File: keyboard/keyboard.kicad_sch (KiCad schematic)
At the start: 64 parts, among them J1 Conn_01x04, J2 Conn_01x04, SW1 SW_Push, SW10 SW_Push, SW11 SW_Push, SW12 SW_Push, SW13 SW_Push, SW14 SW_Push, SW15 SW_Push, SW16 SW_Push, SW17 SW_Push, SW18 SW_Push, SW19 SW_Push, SW2 SW_Push, SW20 SW_Push, SW21 SW_Push, SW3 SW_Push, SW4 SW_Push, SW5 SW_Push, SW6 SW_Push, SW7 SW_Push, SW8 SW_Push, SW9 SW_Push, U1 AP2127K-3.3, U2 USBLC6-2SC6, U3 STM32F072CBTx

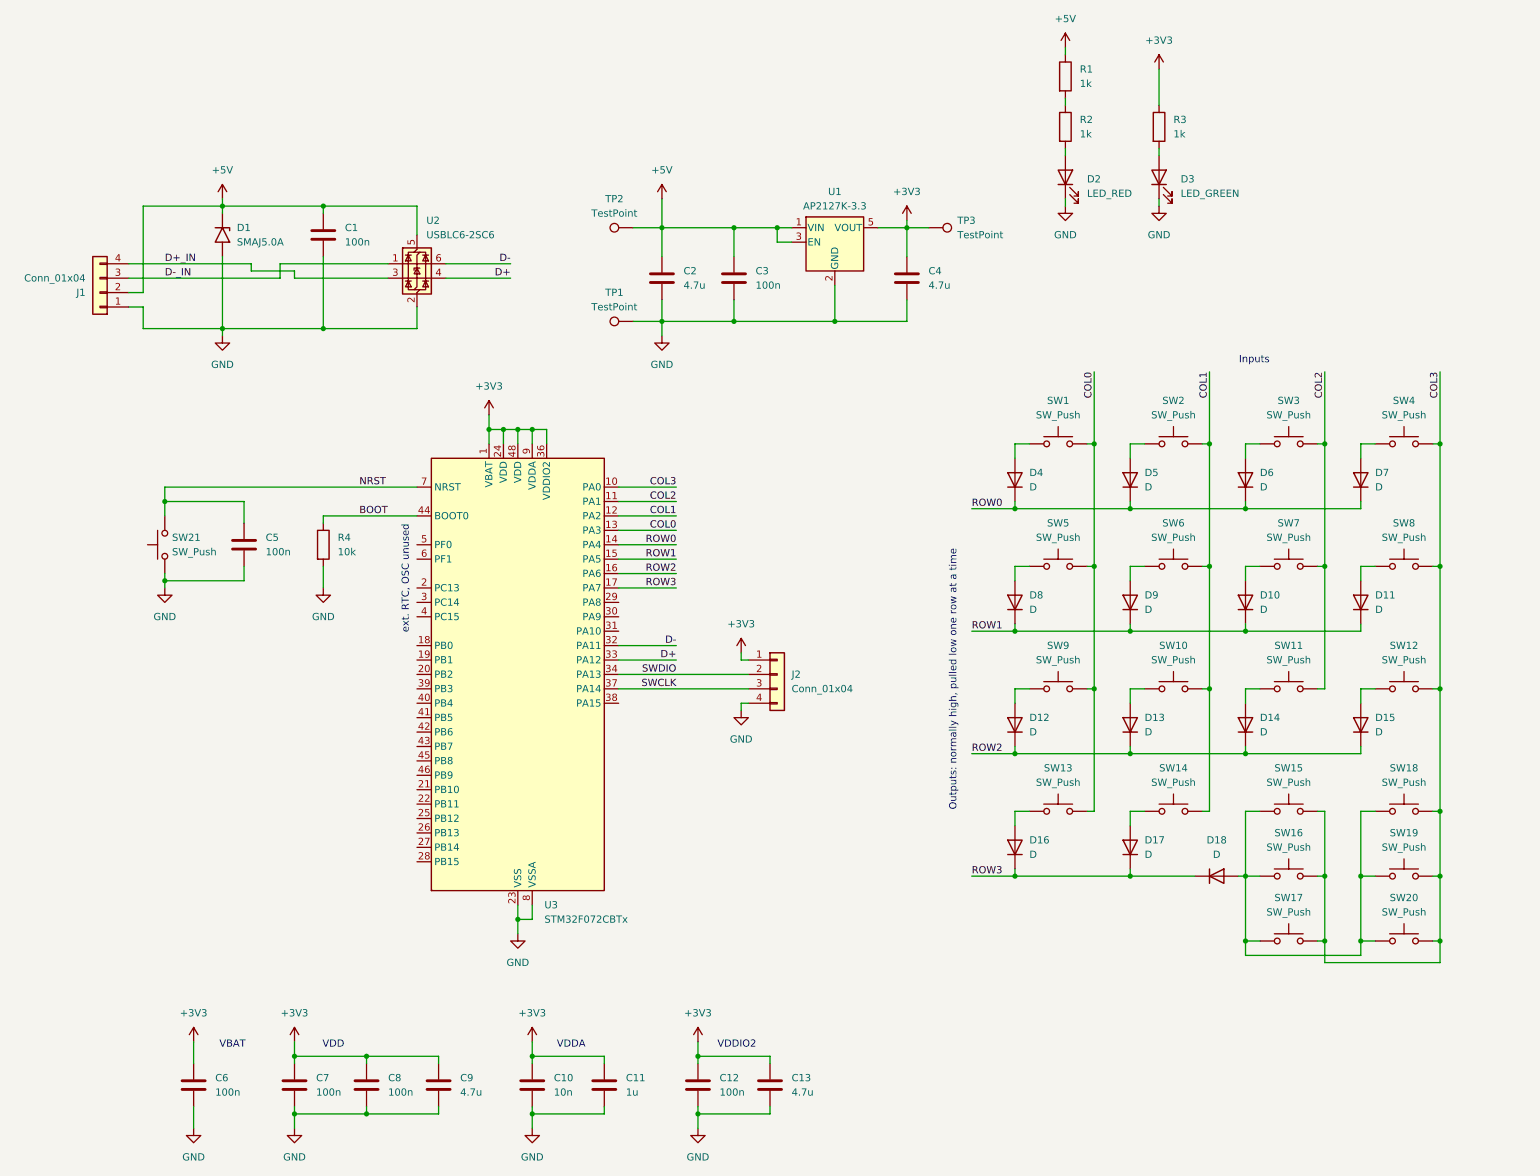
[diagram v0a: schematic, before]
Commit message: Some routing.
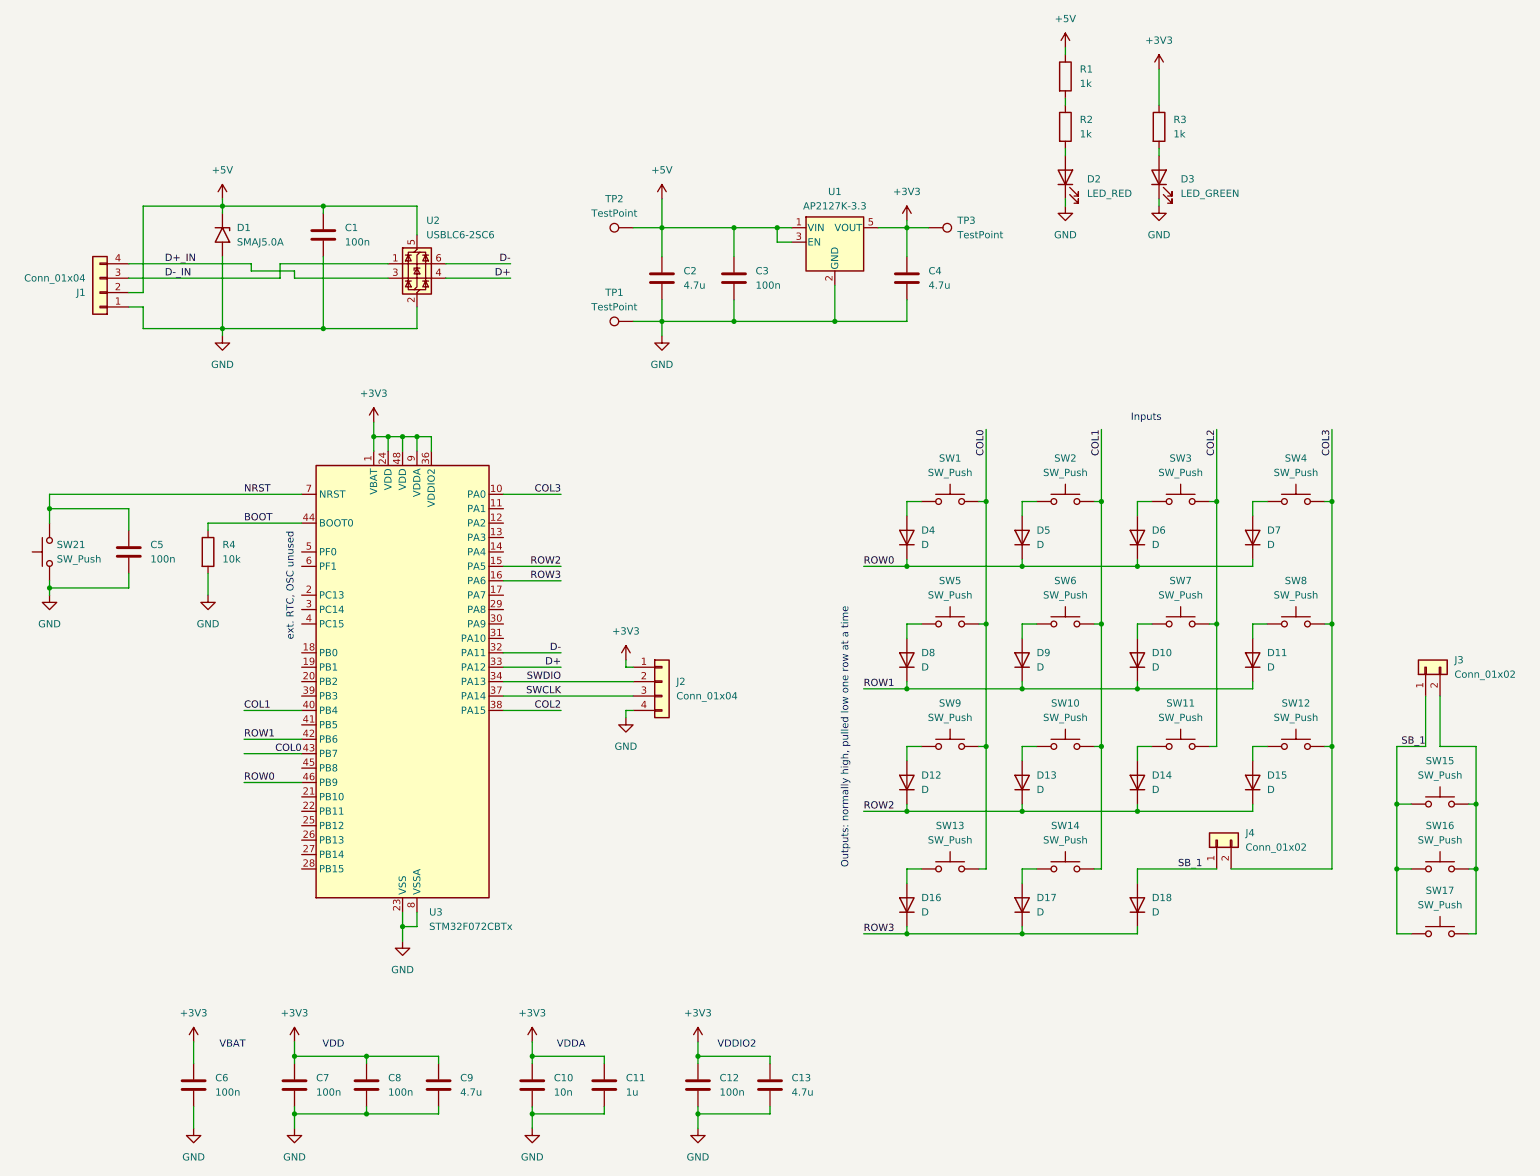
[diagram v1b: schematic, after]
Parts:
- removed SW18, SW19, SW20: SW_Push, PCM_marbastlib-mx:SW_MX_HS_KS-2P02B01-01_1.5u, symbol Switch:SW_Push
- added J3, J4: Conn_01x02, symbol Connector_Generic:Conn_01x02
- J1: footprint Connector_Wire:SolderWire-0.25sqmm_1x04_P4.5mm_D0.65mm_OD2mm_Relief -> (none)
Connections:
- net COL0: now also U3.43 (PB7); no longer U3.13 (PA3)
- net COL1: now also U3.40 (PB4); no longer U3.12 (PA2)
- net COL2: now also U3.38 (PA15); no longer U3.11 (PA1)
- net COL3: now also J4.2 (Pin_2); no longer SW15.2, SW16.2, SW17.2
- net ROW0: now also U3.46 (PB9); no longer U3.14 (PA4)
- net ROW1: now also U3.42 (PB6); no longer U3.15 (PA5)
- net ROW2: now also U3.15 (PA5); no longer U3.16 (PA6)
- net ROW3: now also U3.16 (PA6); no longer U3.17 (PA7)
- net SB_1: now reaches D18.2 (A), SW15.1, SW16.1, SW17.1
- net SB_1: now also J3.1 (Pin_1), J4.1 (Pin_1)
- new net: J3.2 (Pin_2), SW15.2, SW16.2, SW17.2
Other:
- moved on the sheet: C5, D10, D11, D12, D13, D14, D15, D16, D17, D18, D4, D5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
